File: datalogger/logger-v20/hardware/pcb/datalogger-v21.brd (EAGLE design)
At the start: 76.2 x 68.6 mm, 68 parts, among them J10 MF-CON-2.54mm-01x03, J11 MF-CON-2.54mm-01x02, J2 U.FL, J3 CON_01X02SCREW_0.2", J4 ANTENNA_SMA_EDGE, J5 MF-CON-2.54mm-01x03, J6 MF-CON-2.54mm-01x03, J7 MF-CON-2.54mm-01x03, J8 MF-CON-2.54mm-01x03, J9 MF-CON-2.54mm-01x03, Q1 mfet-n, Q2 NFET, Q3 MOSFET-NCHANNELSOT23-3, Q4 MOSFET-NCHANNELSOT23-3, SW1 MF-SW-TACT-4.2MM, SW2 SWITCH_SPDT_SMD_ES01MSABE, U1 RFM69HCW-433MHZ, U2 FT232RL-BASIC-SSOP, U3 ATMEGA1284P-SMD-AU, U4 DS3231M, U5 MCP1703A-500_SOT23-3, U6 TPS62162, Y1 8MHZ

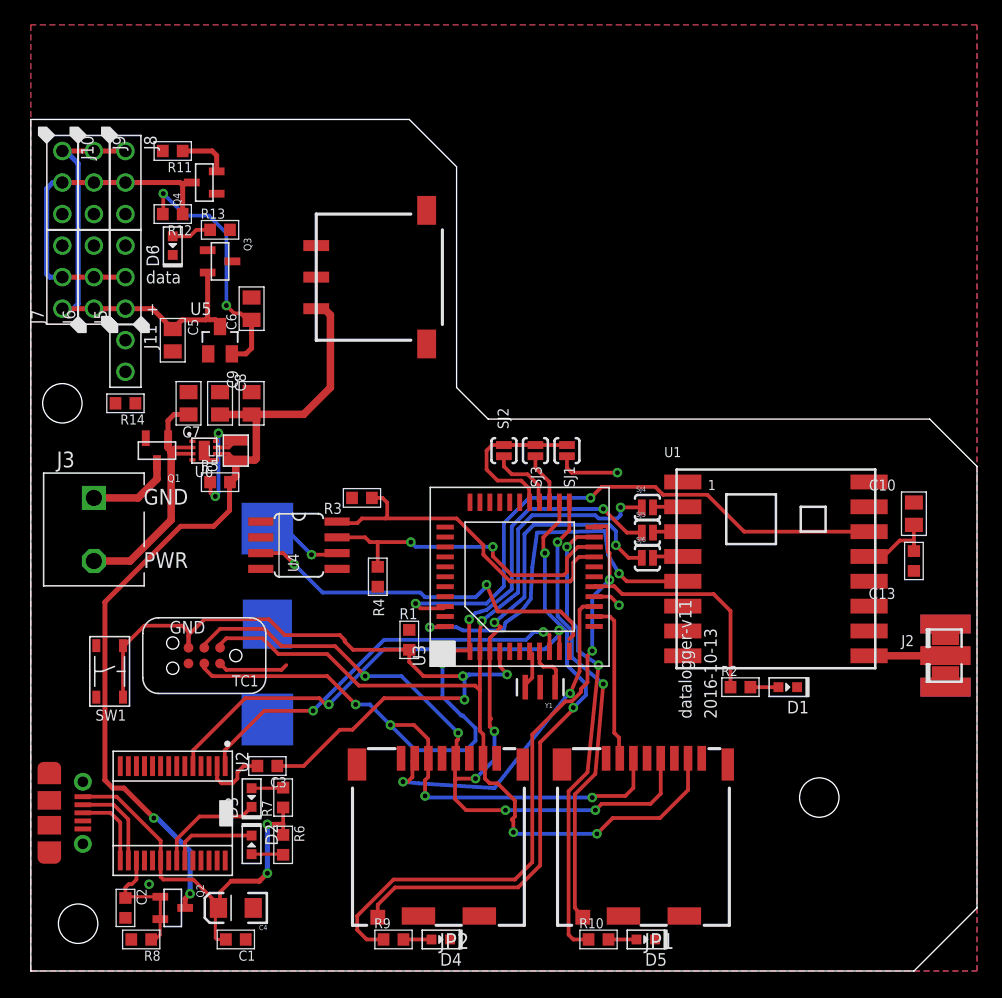
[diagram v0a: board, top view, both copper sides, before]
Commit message: ...
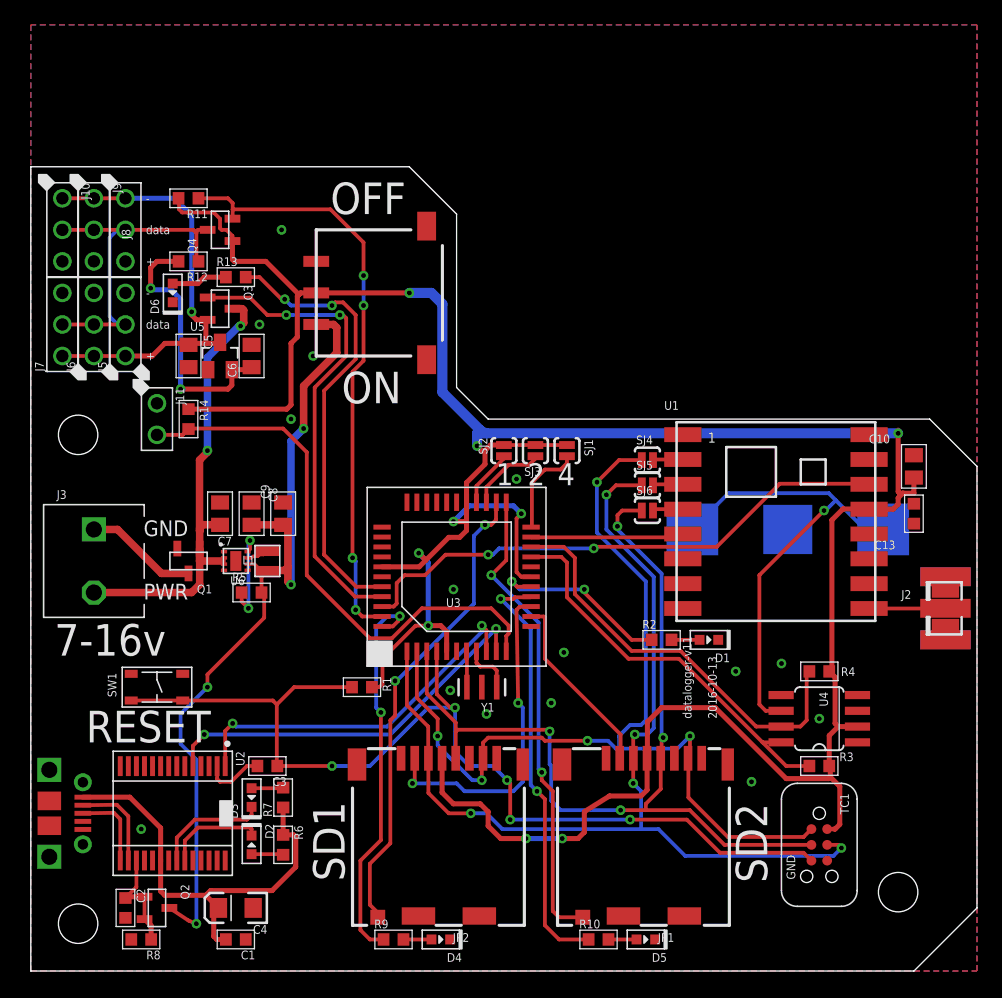
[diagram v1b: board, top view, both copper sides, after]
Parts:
- moved TC1 51.8 mm to (63.5, 10.2), turned to 270 degrees
- moved U4 44.2 mm to (63.5, 20.3), turned to 90 degrees
- moved R3 42.7 mm to (63.5, 16.5), turned to 0 degrees
- moved BAT1 42.6 mm to (61.0, 35.6), turned to 0 degrees
- moved R4 36.4 mm to (63.5, 24.1), turned to 0 degrees
- moved C7 9.25 mm to (15.2, 36.8)
- moved C8 9.25 mm to (17.8, 36.8)
- moved C9 9.25 mm to (20.3, 36.8)
- moved R5 9.25 mm to (17.8, 30.5)
- moved L1 9.25 mm to (19.1, 33.0)
- moved Q1 9.25 mm to (12.7, 33.0)
- moved U6 9.25 mm to (16.5, 33.0)
- moved D1 7.41 mm to (54.6, 26.7)
- moved R2 7.41 mm to (50.8, 26.7)
- moved J11 5.68 mm to (10.2, 44.5)
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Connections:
- net GND: now also J1.P$5, J1.P$6
- net NET_SEL_4: now also U3.22; no longer U3.15
- net RF_CS: now also U3.21; no longer U3.44
- net SD_LED_0: now also U3.15; no longer U3.21
- net SD_LED_1: now also U3.44; no longer U3.22
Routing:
- net 3V3: track 28.7 -> 236.2 mm, vias 0 -> 9
- net RAIN_INT: track 0.00 -> 45.1 mm
- net SDI_DATA_3V3: track 4.17 -> 48.2 mm, vias 0 -> 4
- net SDI_EN: track 0.00 -> 39.0 mm, vias 0 -> 2
- net SDI_LED: track 0.00 -> 36.8 mm, vias 0 -> 2
- net N$10: track 6.53 -> 38.8 mm
- net INT0: track 30.3 -> 0.00 mm, vias 2 -> 0
- net RST: track 63.0 -> 82.7 mm, vias 3 -> 5
- net SD_LED_1: track 50.5 -> 31.6 mm
- net RF_CS: track 30.8 -> 12.5 mm, vias 2 -> 0
- net V_BAT: track 21.1 -> 39.0 mm, vias 0 -> 2
- net SCK: track 86.1 -> 73.4 mm, vias 8 -> 4
- net CARD_DETECT_1: track 48.1 -> 38.3 mm
- net SDA: track 26.0 -> 34.1 mm, vias 2 -> 0
- net RX0: track 37.1 -> 31.8 mm
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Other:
- board size 76.2 x 68.6 mm -> 76.2 x 64.8 mm
- board text added: "1"
- board text added: "2"
- board text added: "4"
- board text added: "7-16v"
- board text added: "OFF"
- board text added: "ON"
- board text added: "RESET"
- board text added: "SD1"
- board text added: "SD2"
